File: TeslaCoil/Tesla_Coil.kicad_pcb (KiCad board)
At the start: 4 copper layers, 48 x 25 mm, 2 parts, among them Q1 Q_NPN_BCE

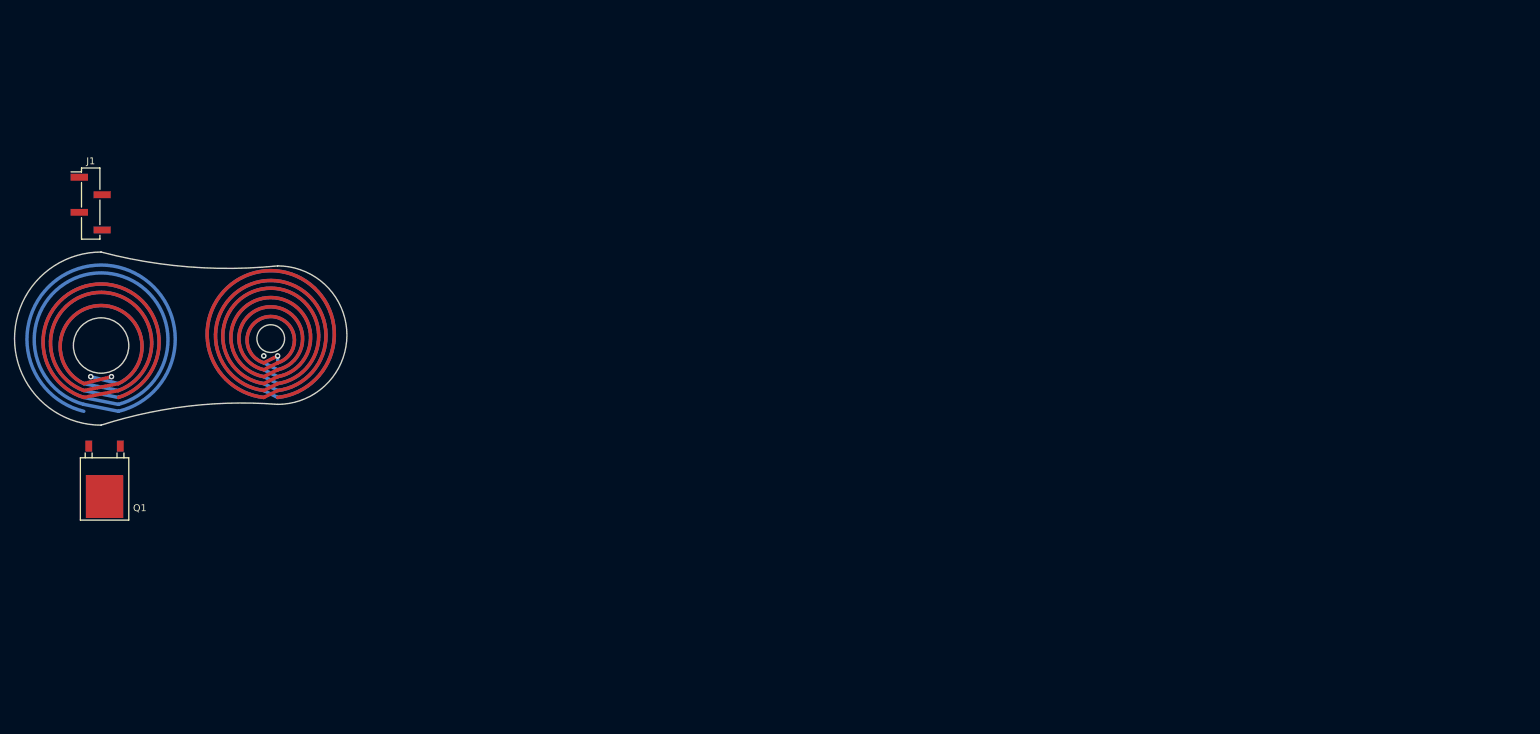
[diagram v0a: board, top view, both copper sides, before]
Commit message: save
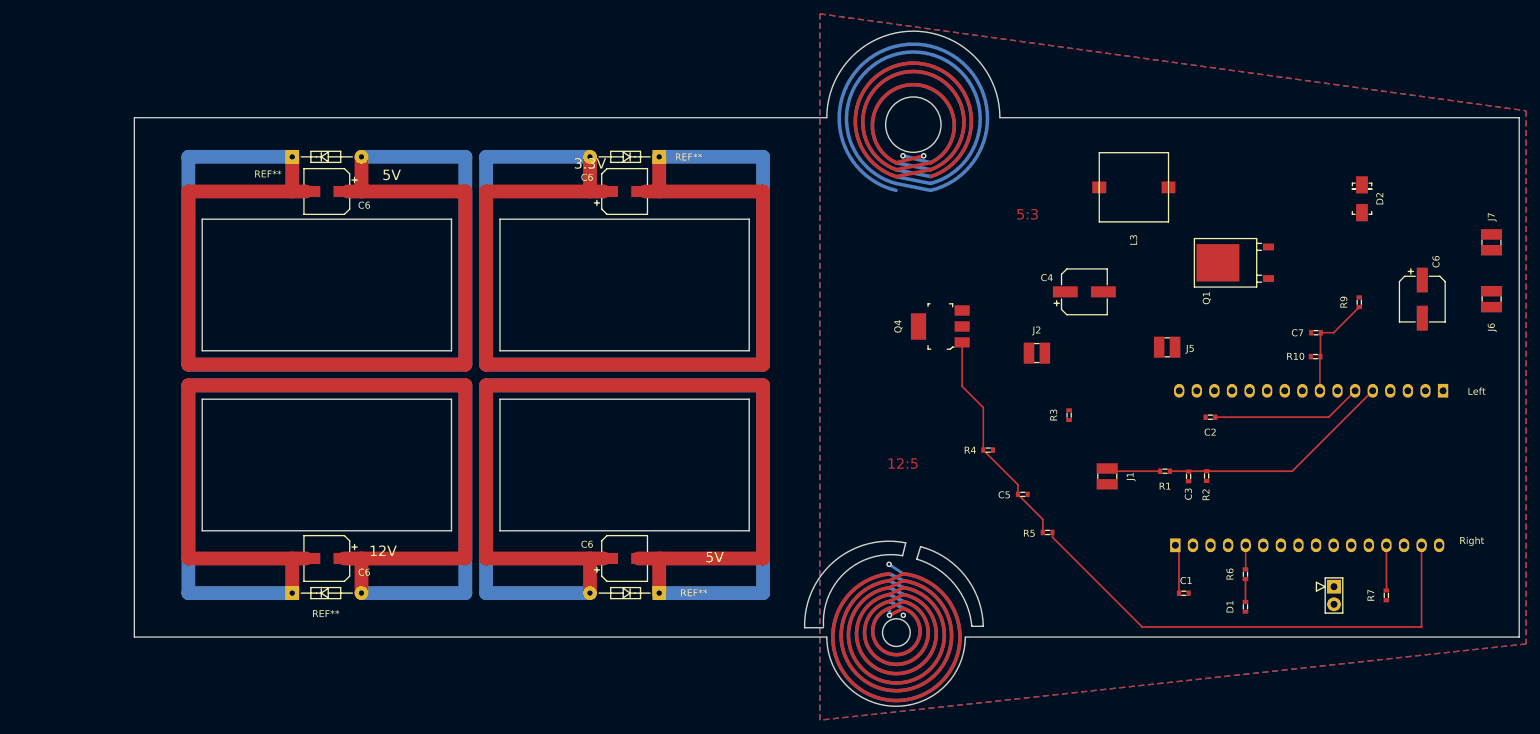
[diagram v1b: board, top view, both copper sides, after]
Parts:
- added C1: 0.1uF, digikey-footprints:0603, F.Cu at (262.8, 147.0)
- added C2: 0.1uF, digikey-footprints:0603, F.Cu at (266.6, 121.6)
- added C3: 0.1uF, digikey-footprints:0603, F.Cu at (263.4, 130.1)
- added C4: 100uF, ESP32-footprints-Lib:Cpol-6.3x7.7, F.Cu at (248.4, 103.5)
- added C5: 1nF, digikey-footprints:0603, F.Cu at (239.5, 132.7)
- added C6: 220uF, ESP32-footprints-Lib:Cpol-6.3x7.7, F.Cu at (139.0, 89.0)
- added C6: 220uF, ESP32-footprints-Lib:Cpol-6.3x7.7, F.Cu at (182.0, 142.0)
- added C6: 220uF, ESP32-footprints-Lib:Cpol-6.3x7.7, F.Cu at (297.2, 104.5)
- added C6: 220uF, ESP32-footprints-Lib:Cpol-6.3x7.7, F.Cu at (139.0, 142.0)
- added C6: 220uF, ESP32-footprints-Lib:Cpol-6.3x7.7, F.Cu at (182.0, 89.0)
- added C7: 0.1uF, digikey-footprints:0603, F.Cu at (281.9, 109.4)
- added D1: COMMS, digikey-footprints:0603, F.Cu at (271.7, 149.0)
- added D2: D_Schottky, digikey-footprints:DO-214AC, F.Cu at (288.5, 90.0)
- added J2: SOLAR_OUTPUT, digikey-footprints:1210, F.Cu at (241.6, 112.3)
- added J3: Left, ESP32-footprints-Lib:PIN16, F.Cu at (279.9, 119.1)
- added J4: Right, ESP32-footprints-Lib:PIN16, F.Cu at (281.9, 138.8)
- added J5: 5V, digikey-footprints:1210, F.Cu at (260.4, 111.5)
- added J6: BATTERY_INPUT, digikey-footprints:1210, F.Cu at (307.2, 104.5)
- added J7: BATTERY_OUTPUT, digikey-footprints:1210, F.Cu at (307.2, 96.3)
- added L3: 33uH, ESP32-footprints-Lib:7447779139, F.Cu at (255.6, 88.4)
- added Q4: IRFIZ44N, digikey-footprints:SOT-223, F.Cu at (227.6, 108.5)
- added R1: 10k, digikey-footprints:0603, F.Cu at (260.1, 129.4)
- added R10: 560R, digikey-footprints:0603, F.Cu at (281.8, 112.8)
- added R2: 560R, digikey-footprints:0603, F.Cu at (266.1, 130.1)
- added R3: 0.005R, digikey-footprints:0603, F.Cu at (246.2, 121.3)
- added R4: 10k, digikey-footprints:0603, F.Cu at (234.5, 126.3)
- added R5: 100R, digikey-footprints:0603, F.Cu at (243.1, 138.2)
- added R6: 560R, digikey-footprints:0603, F.Cu at (271.7, 144.3)
- added R7: 220R, digikey-footprints:0603, F.Cu at (292.0, 147.3)
- added R9: 10k, digikey-footprints:0603, F.Cu at (288.1, 105.0)
- added REF**: Diode_DO-35_P10mm, digikey-footprints:Diode_DO-35_P10mm, F.Cu at (187.0, 84.0)
- added REF**: Diode_DO-35_P10mm, digikey-footprints:Diode_DO-35_P10mm, F.Cu at (134.0, 147.0)
- added REF**: Diode_DO-35_P10mm, digikey-footprints:Diode_DO-35_P10mm, F.Cu at (134.0, 84.0)
- added REF**: Diode_DO-35_P10mm, digikey-footprints:Diode_DO-35_P10mm, F.Cu at (187.0, 147.0)
- added RX1: GPIO, ESP32-footprints-Lib:PIN2, F.Cu at (284.4, 147.3)
- J1: renamed from J?; value GPIOs -> SOLAR_INPUT; footprint Connector_PinHeader_2.54mm:PinHeader_1x04_P2.54mm_Vertical_SMD_Pin1Left -> digikey-footprints:1210
- moved Q1 164.3 mm to (267.7, 99.3), turned to 90 degrees
- moved J1 152.0 mm to (251.7, 130.1), turned to -90 degrees
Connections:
- J1 pad 1: 12v -> Net-(IC1-Pad8)
- J1 pad 2: 5v -> GND
- Q1 pad 3: Net-(BT1-Pad1) -> Bat+
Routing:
- net PWM: track 0.00 -> 71.2 mm
- net U_Sol: track 0.00 -> 34.1 mm
- net Net-(C5-Pad2): track 0.00 -> 32.3 mm
- net I_Sol: track 0.00 -> 21.8 mm
- net U_Bat: track 0.00 -> 15.5 mm
- net Net-(IC1-Pad8): track 0.00 -> 8.51 mm
- net +3V3: track 0.00 -> 7.15 mm
- net Net-(J4-Pad13): track 0.00 -> 6.75 mm
- net Net-(J4-Pad5): track 0.00 -> 3.50 mm
- net Net-(D1-Pad2): track 0.00 -> 3.30 mm
- net GND: vias 0 -> 3
- net (no net): vias 4 -> 2
- added copper zone on B.Cu, net GND
- added copper zone on F.Cu, net GND
- added copper zone on In1.Cu, net GND
- added copper zone on In2.Cu, net GND
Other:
- board size 48 x 25 mm -> 200 x 97.5 mm
- board text added: "12:5"
- board text added: "12V"
- board text added: "3.3V"
- board text added: "5:3"
- board text added: "5V"
